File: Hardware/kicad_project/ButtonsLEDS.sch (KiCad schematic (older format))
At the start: 100 parts

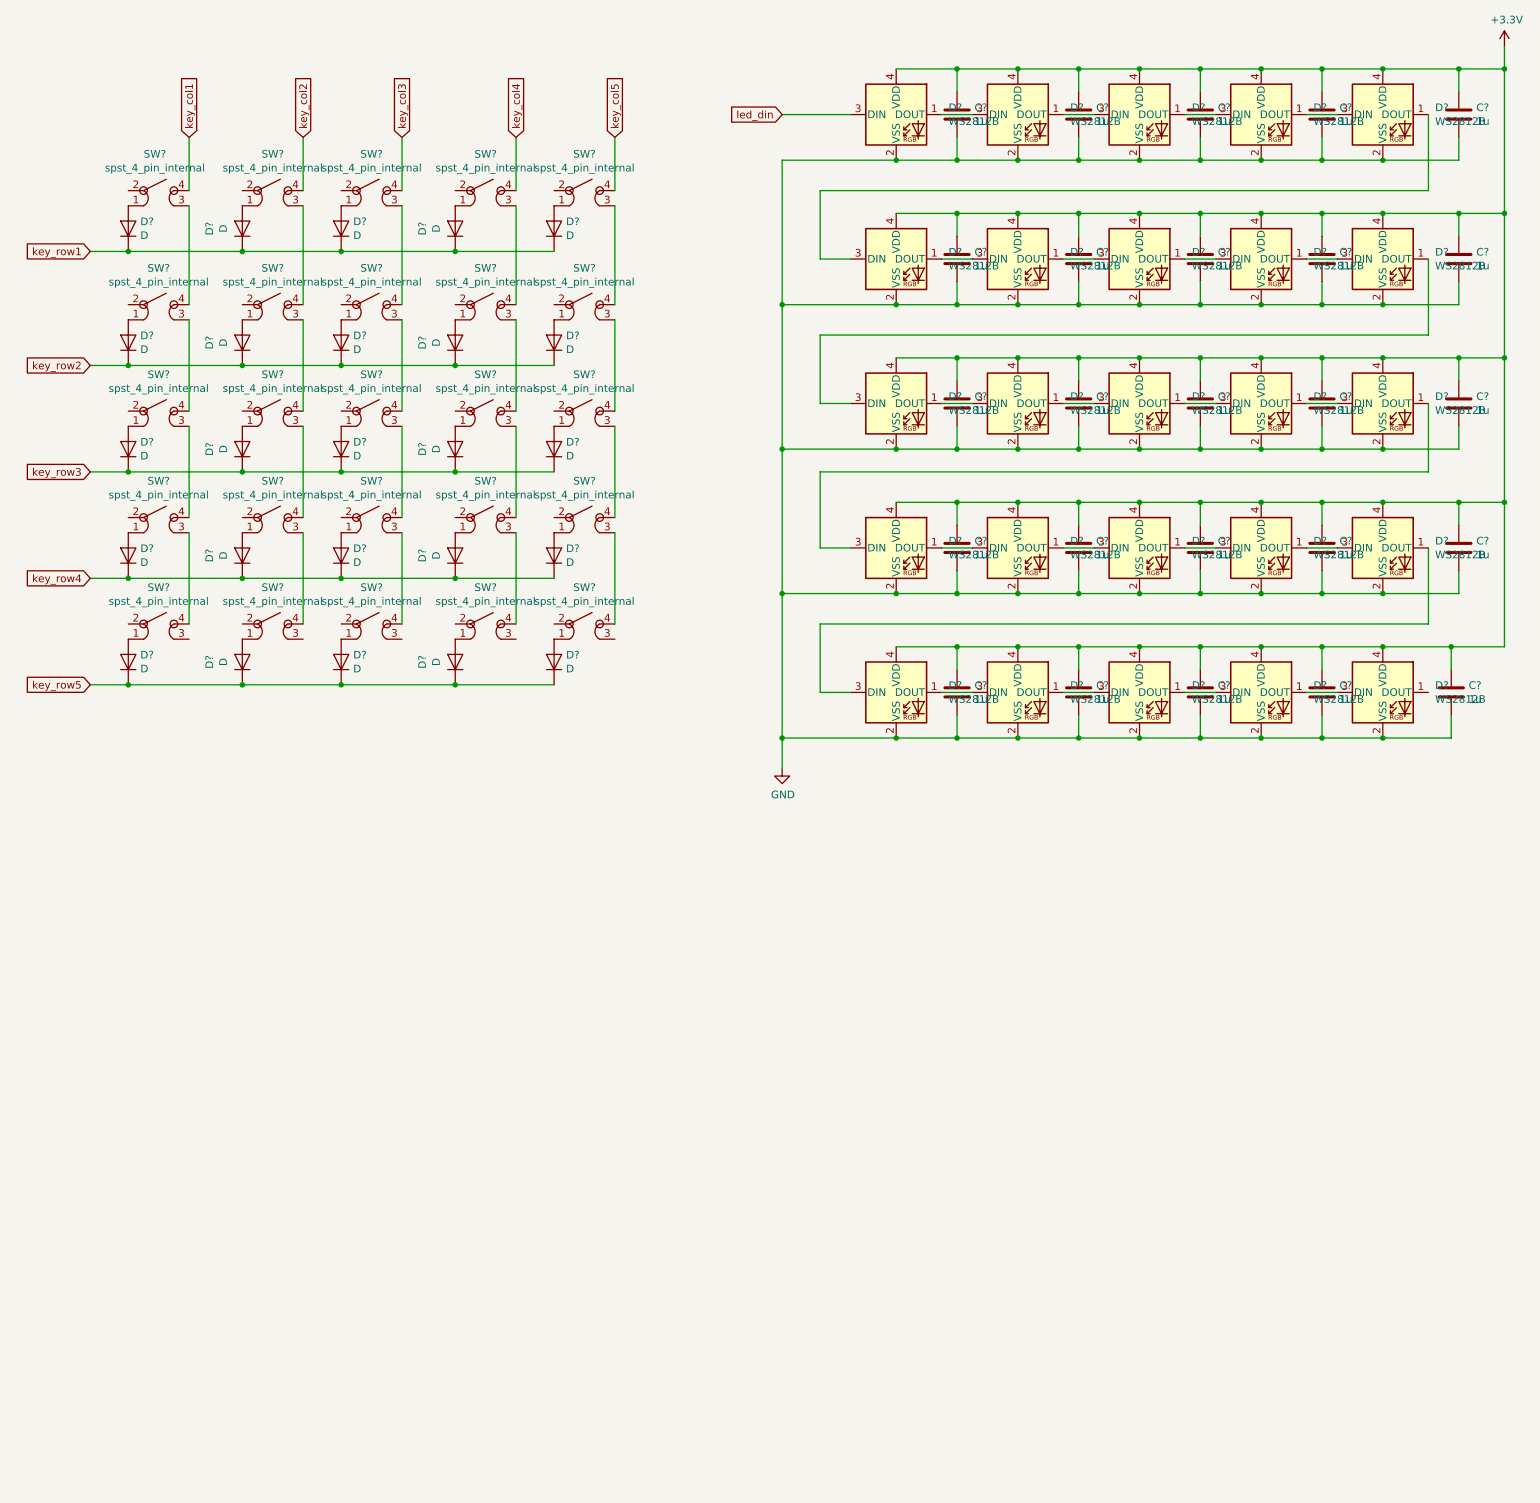
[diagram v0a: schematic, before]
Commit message: update project with corrected schematic / pcb
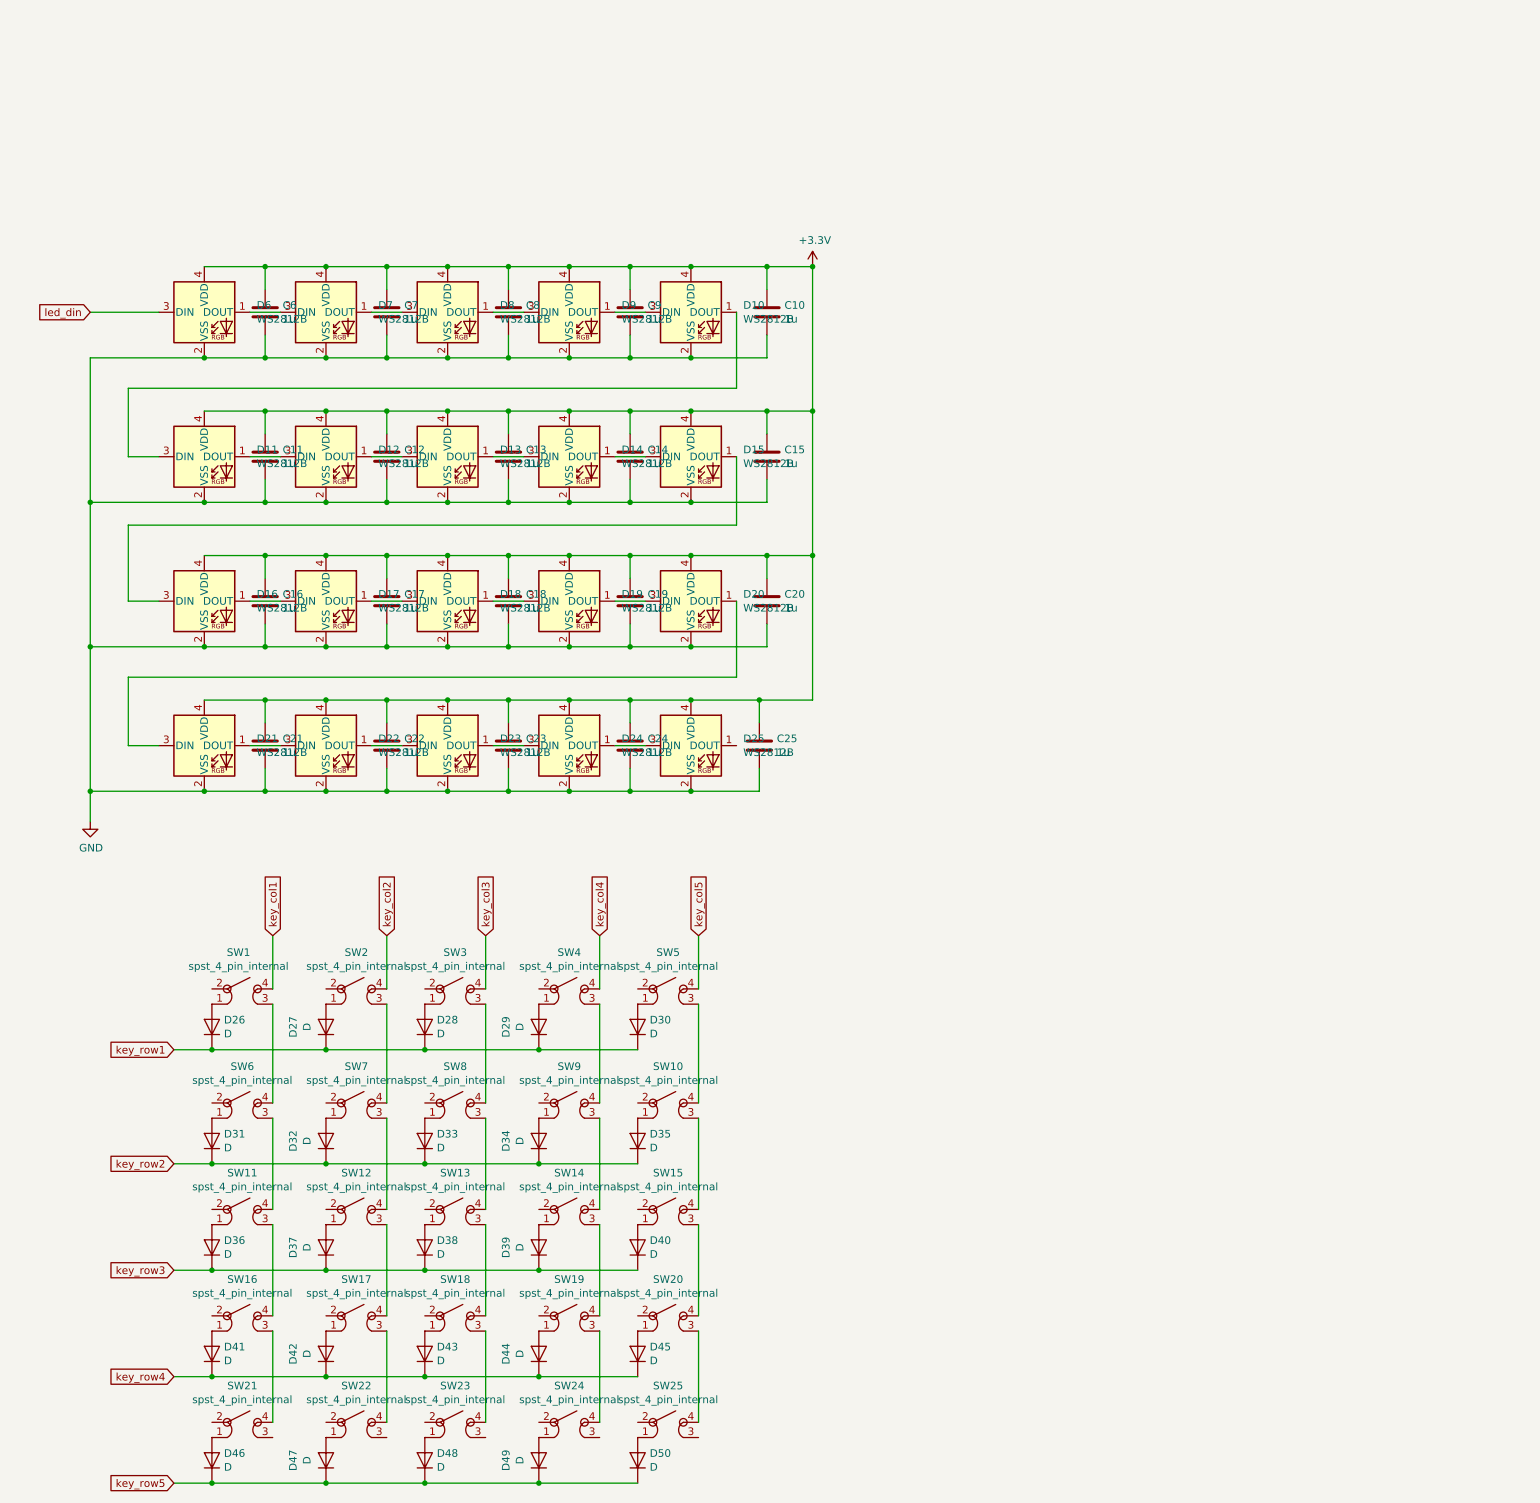
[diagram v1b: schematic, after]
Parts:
- removed C? (x25): 1u, RandomJunk:C_0402_NoSilk, symbol Device:C
- removed D? (x25): D, RandomJunk:D_SOD-323F_less_silk, symbol Device:D
- removed D? (x25): WS2812B, RandomJunk:ws2812b-2020-lightpipe, symbol customLibrary:WS2812B-2020
- removed SW? (x25): spst_4_pin_internal, RandomJunk:ts1102_smallerpads_buttonhole, symbol customLibrary:spst_4_pin_internal
- added C10, C11, C12, C13, C14, C15, C16, C17, C18, C19, C20, C21, C22, C23, C24, C25, C6, C7, C8, C9: 1u, Capacitors_SMD:C_0402_NoSilk, symbol Device:C
- added D10, D11, D12, D13, D14, D15, D16, D17, D18, D19, D20, D21, D22, D23, D24, D25, D6, D7, D8, D9: WS2812B, RandomJunk:ws2812b-2020-lightpipe, symbol customLibrary:WS2812B-2020
- added D26, D27, D28, D29, D30, D31, D32, D33, D34, D35, D36, D37, D38, D39, D40, D41, D42, D43, D44, D45, D46, D47, D48, D49, D50: D, RandomJunk:D_SOD-323F_less_silk, symbol Device:D
- added SW1, SW10, SW11, SW12, SW13, SW14, SW15, SW16, SW17, SW18, SW19, SW2, SW20, SW21, SW22, SW23, SW24, SW25, SW3, SW4, SW5, SW6, SW7, SW8, SW9: spst_4_pin_internal, RandomJunk:ts1102_smallerpads_buttonhole, symbol customLibrary:spst_4_pin_internal
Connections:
- net +3V3: now also C10.1, C11.1, C12.1, C13.1, C14.1, C15.1, C16.1, C17.1, C18.1, C19.1, C20.1, C21.1, C22.1, C23.1, C24.1, C25.1, C6.1, C7.1, C8.1, C9.1, D10.4 (VDD), D11.4 (VDD), D12.4 (VDD), D13.4 (VDD), D14.4 (VDD), D15.4 (VDD), D16.4 (VDD), D17.4 (VDD), D18.4 (VDD), D19.4 (VDD), D20.4 (VDD), D21.4 (VDD), D22.4 (VDD), D23.4 (VDD), D24.4 (VDD), D25.4 (VDD), D6.4 (VDD), D7.4 (VDD), D8.4 (VDD), D9.4 (VDD)
- net GND: now also C10.2, C11.2, C12.2, C13.2, C14.2, C15.2, C16.2, C17.2, C18.2, C19.2, C20.2, C21.2, C22.2, C23.2, C24.2, C25.2, C6.2, C7.2, C8.2, C9.2, D10.2 (VSS), D11.2 (VSS), D12.2 (VSS), D13.2 (VSS), D14.2 (VSS), D15.2 (VSS), D16.2 (VSS), D17.2 (VSS), D18.2 (VSS), D19.2 (VSS), D20.2 (VSS), D21.2 (VSS), D22.2 (VSS), D23.2 (VSS), D24.2 (VSS), D25.2 (VSS), D6.2 (VSS), D7.2 (VSS), D8.2 (VSS), D9.2 (VSS)
- net key_col1: now also SW1.4
- net key_col2: now also SW2.4
- net key_col3: now also SW3.4
- net key_col4: now also SW4.4
- net key_col5: now also SW5.4
- net key_row1: now also D26.1 (K), D27.1 (K), D28.1 (K), D29.1 (K), D30.1 (K)
- net key_row2: now also D31.1 (K), D32.1 (K), D33.1 (K), D34.1 (K), D35.1 (K)
- net key_row3: now also D36.1 (K), D37.1 (K), D38.1 (K), D39.1 (K), D40.1 (K)
- net key_row4: now also D41.1 (K), D42.1 (K), D43.1 (K), D44.1 (K), D45.1 (K)
- net key_row5: now also D46.1 (K), D47.1 (K), D48.1 (K), D49.1 (K), D50.1 (K)
- net led_din: now also D6.3 (DIN)
- new net: D50.2 (A), SW25.1
- new net: SW20.3, SW25.4
- new net: D49.2 (A), SW24.1
- new net: SW19.3, SW24.4
- new net: D48.2 (A), SW23.1
- new net: SW18.3, SW23.4
- new net: D47.2 (A), SW22.1
- new net: SW17.3, SW22.4
- new net: D46.2 (A), SW21.1
- new net: SW16.3, SW21.4
- new net: D45.2 (A), SW20.1
- new net: SW15.3, SW20.4
- new net: D44.2 (A), SW19.1
- new net: SW14.3, SW19.4
- new net: D43.2 (A), SW18.1
- new net: SW13.3, SW18.4
- new net: D42.2 (A), SW17.1
- new net: SW12.3, SW17.4
- new net: D41.2 (A), SW16.1
- new net: SW11.3, SW16.4
- new net: D40.2 (A), SW15.1
- new net: SW10.3, SW15.4
- new net: D39.2 (A), SW14.1
- new net: SW14.4, SW9.3
- new net: D38.2 (A), SW13.1
- new net: SW13.4, SW8.3
- new net: D37.2 (A), SW12.1
- new net: SW12.4, SW7.3
- new net: D36.2 (A), SW11.1
- new net: SW11.4, SW6.3
- new net: D35.2 (A), SW10.1
- new net: SW10.4, SW5.3
- new net: D34.2 (A), SW9.1
- new net: SW4.3, SW9.4
- new net: D33.2 (A), SW8.1
- new net: SW3.3, SW8.4
- new net: D32.2 (A), SW7.1
- new net: SW2.3, SW7.4
- new net: D31.2 (A), SW6.1
- new net: SW1.3, SW6.4
- new net: D30.2 (A), SW5.1
- new net: D29.2 (A), SW4.1
- new net: D28.2 (A), SW3.1
- new net: D27.2 (A), SW2.1
- new net: D26.2 (A), SW1.1
- new net: D24.1 (DOUT), D25.3 (DIN)
- new net: D23.1 (DOUT), D24.3 (DIN)
- new net: D22.1 (DOUT), D23.3 (DIN)
- new net: D21.1 (DOUT), D22.3 (DIN)
- new net: D20.1 (DOUT), D21.3 (DIN)
- new net: D19.1 (DOUT), D20.3 (DIN)
- new net: D18.1 (DOUT), D19.3 (DIN)
- new net: D17.1 (DOUT), D18.3 (DIN)
- new net: D16.1 (DOUT), D17.3 (DIN)
- new net: D15.1 (DOUT), D16.3 (DIN)
- new net: D14.1 (DOUT), D15.3 (DIN)
- new net: D13.1 (DOUT), D14.3 (DIN)
- new net: D12.1 (DOUT), D13.3 (DIN)
- new net: D11.1 (DOUT), D12.3 (DIN)
- new net: D10.1 (DOUT), D11.3 (DIN)
- new net: D10.3 (DIN), D9.1 (DOUT)
- new net: D8.1 (DOUT), D9.3 (DIN)
- new net: D7.1 (DOUT), D8.3 (DIN)
- new net: D6.1 (DOUT), D7.3 (DIN)
